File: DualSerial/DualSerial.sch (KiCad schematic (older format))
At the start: 22 parts, among them CN1 DB9 Male, CN2 DB9 Male, J1 COM_A_SELECT, J2 IRQ_A_SELECT, J3 COM_A_SELECT, J4 IRQ_B_SELECT, J5 Bus_ISA_8bit, U1 16550/16C550, U2 GAL16V8, U3 GD75232N, U4 1.8432 MHz, U8 16550/16C550, U9 GD75232N

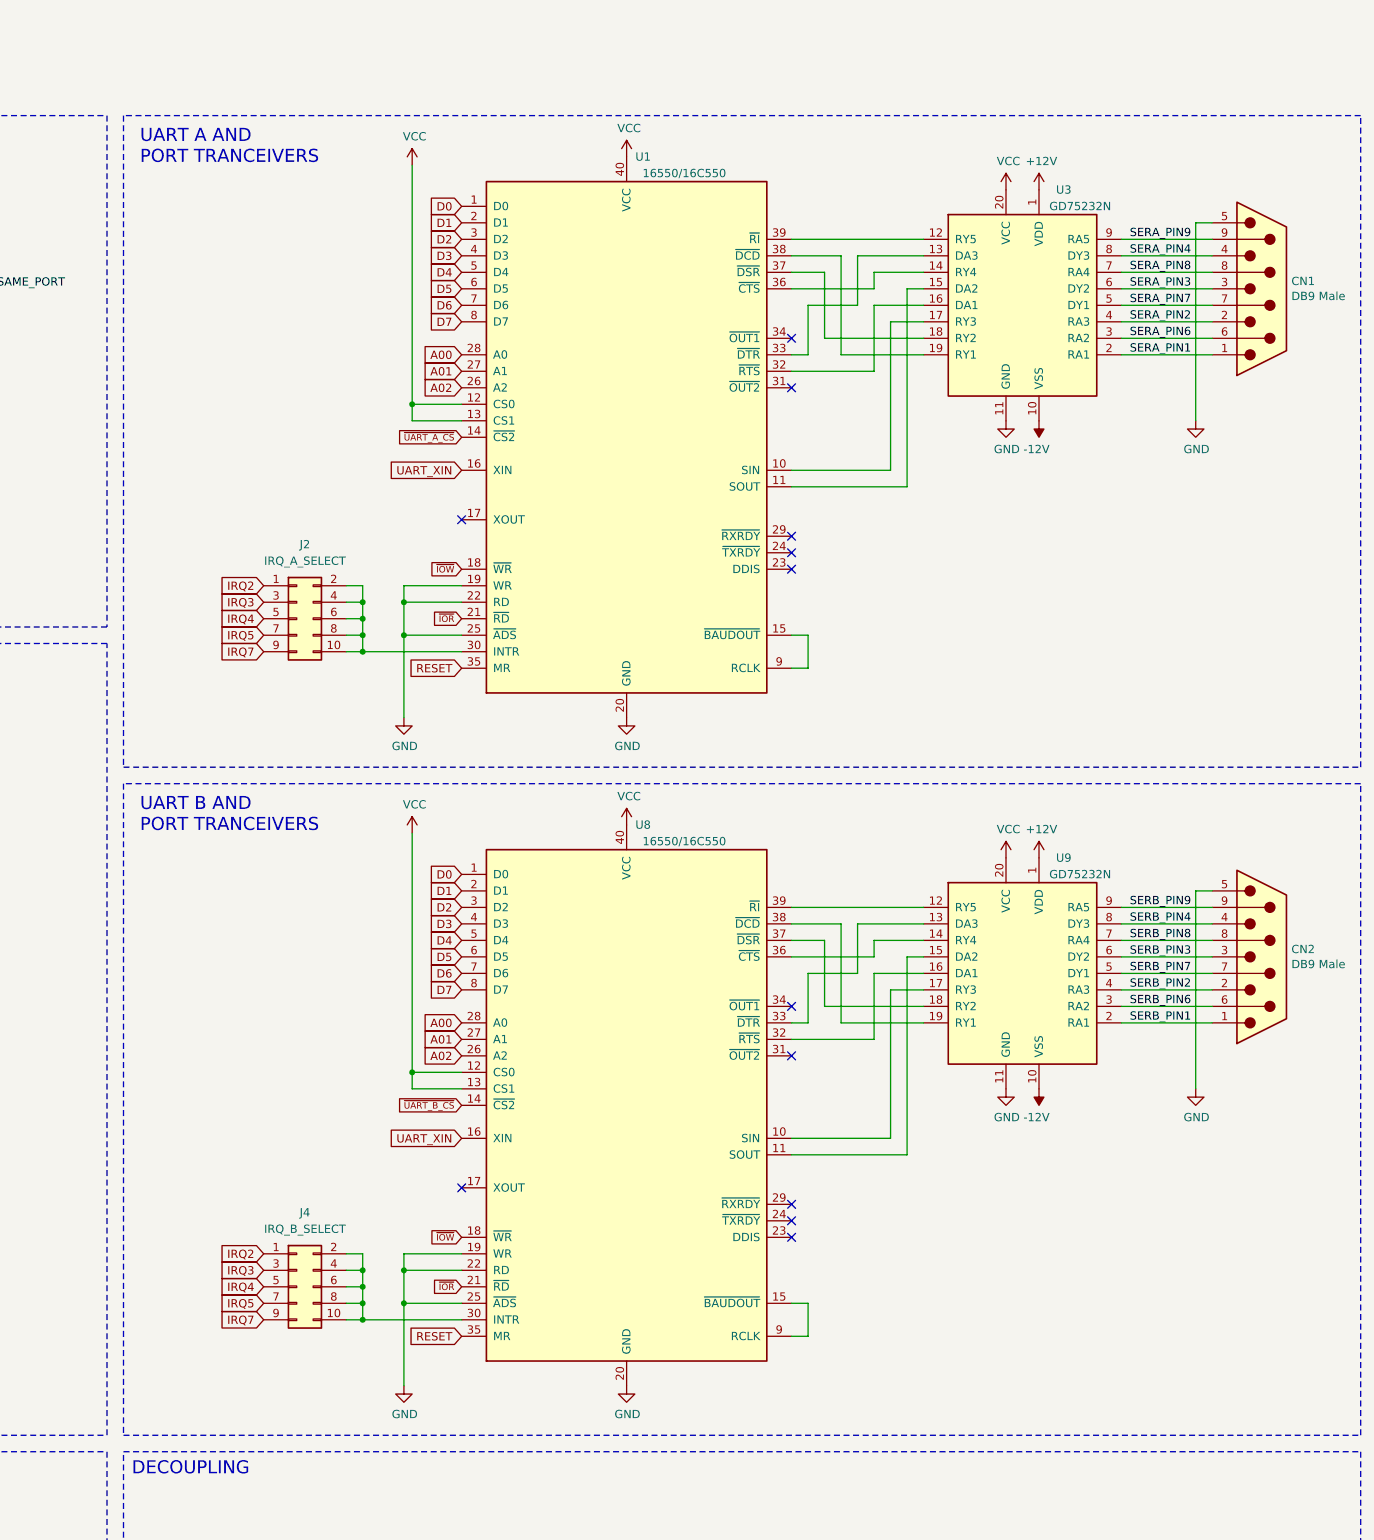
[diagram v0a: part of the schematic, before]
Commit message: DualSerial: More WIP on PCB layout.
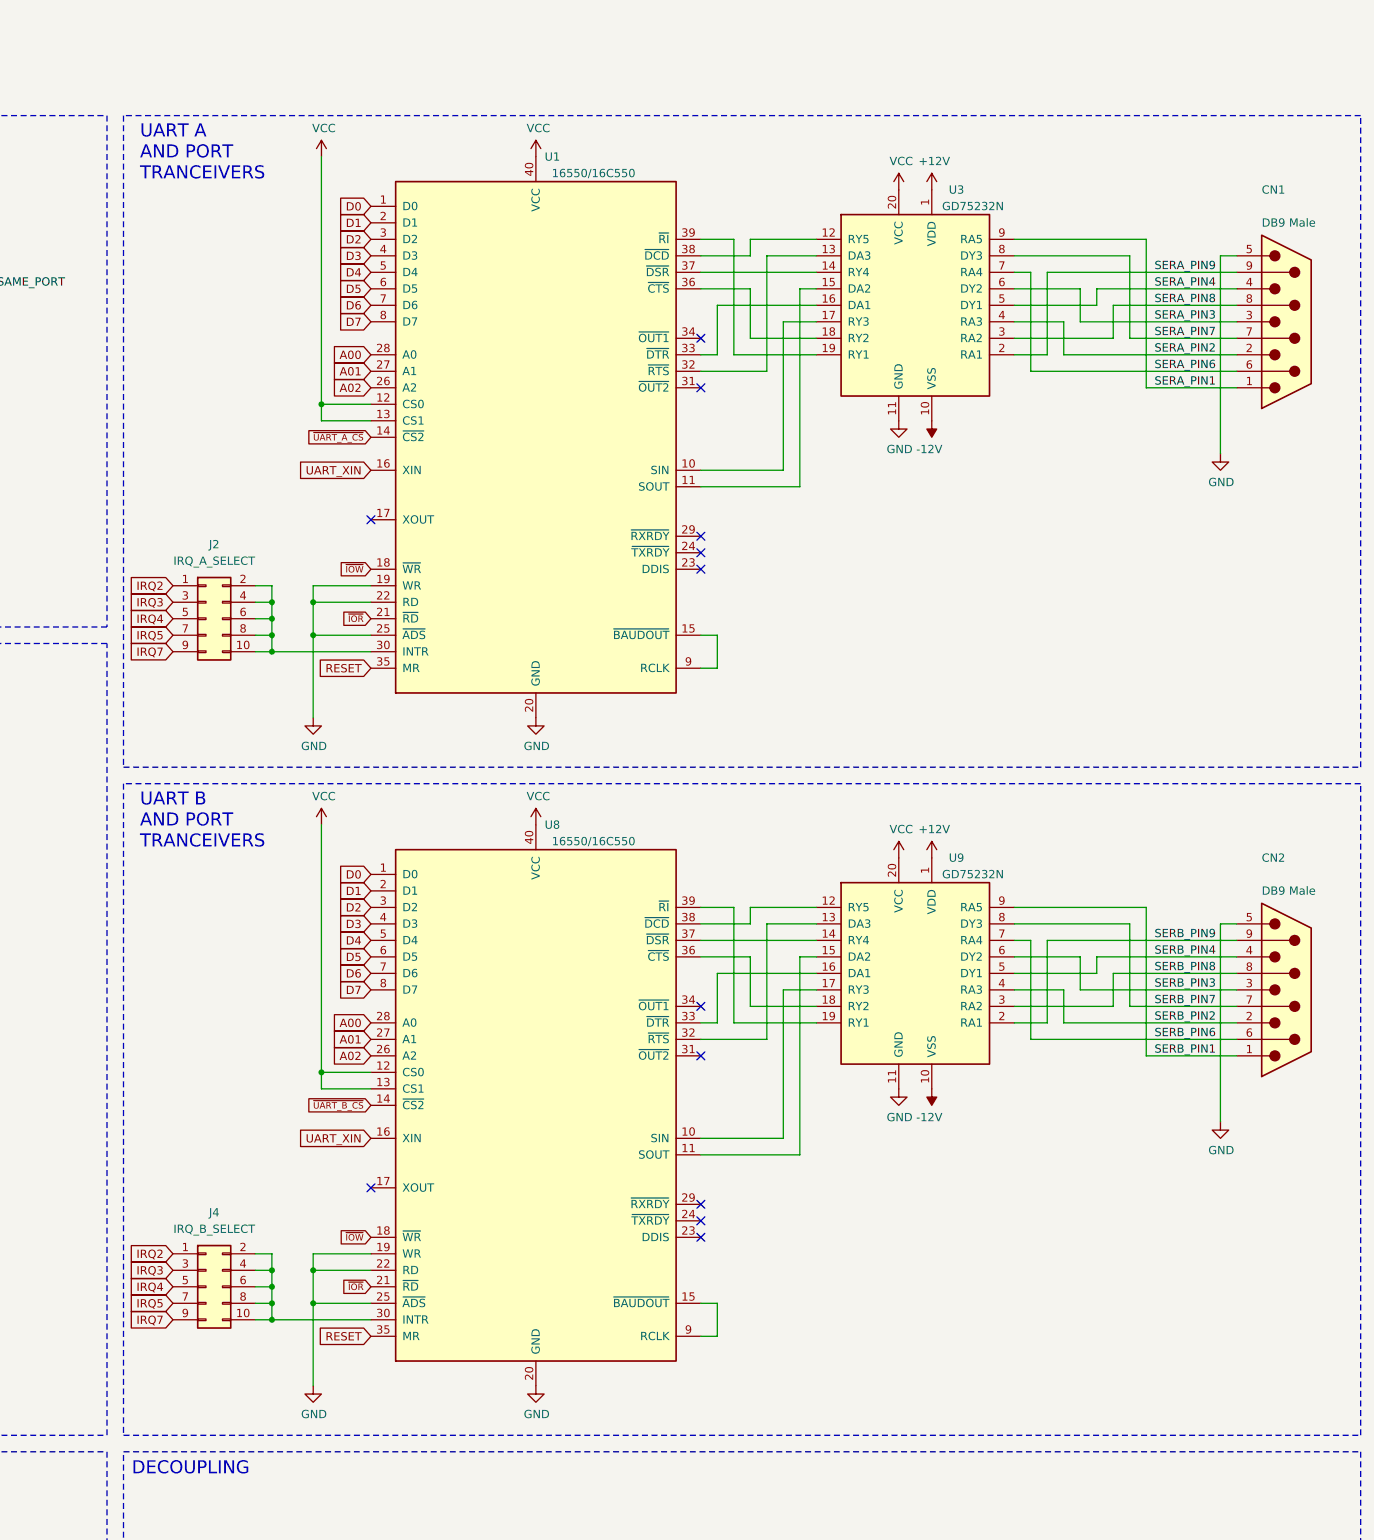
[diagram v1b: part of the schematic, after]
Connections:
- net SERA_PIN1: now also U3.9 (RA5); no longer U3.2 (RA1)
- net SERA_PIN4: now also U3.5 (DY1); no longer U3.8 (DY3)
- net SERA_PIN6: now also U3.7 (RA4); no longer U3.3 (RA2)
- net SERA_PIN7: now also U3.8 (DY3); no longer U3.5 (DY1)
- net SERA_PIN8: now also U3.3 (RA2); no longer U3.7 (RA4)
- net SERA_PIN9: now also U3.2 (RA1); no longer U3.9 (RA5)
- net SERB_PIN1: now also U9.9 (RA5); no longer U9.2 (RA1)
- net SERB_PIN4: now also U9.5 (DY1); no longer U9.8 (DY3)
- net SERB_PIN6: now also U9.7 (RA4); no longer U9.3 (RA2)
- net SERB_PIN7: now also U9.8 (DY3); no longer U9.5 (DY1)
- net SERB_PIN8: now also U9.3 (RA2); no longer U9.7 (RA4)
- net SERB_PIN9: now also U9.2 (RA1); no longer U9.9 (RA5)
- net at U1.32 (~RTS~): now also U3.13 (DA3); no longer U3.16 (DA1)
- net at U1.33 (~DTR~): now also U3.16 (DA1); no longer U3.13 (DA3)
- net at U1.36 (~CTS~): now also U3.18 (RY2); no longer U3.14 (RY4)
- net at U1.37 (~DSR~): now also U3.14 (RY4); no longer U3.18 (RY2)
- net at U1.38 (~DCD~): now also U3.12 (RY5); no longer U3.19 (RY1)
- net at U1.39 (~RI~): now also U3.19 (RY1); no longer U3.12 (RY5)
- net at U8.32 (~RTS~): now also U9.13 (DA3); no longer U9.16 (DA1)
- net at U8.33 (~DTR~): now also U9.16 (DA1); no longer U9.13 (DA3)
- net at U8.36 (~CTS~): now also U9.18 (RY2); no longer U9.14 (RY4)
- net at U8.37 (~DSR~): now also U9.14 (RY4); no longer U9.18 (RY2)
- net at U8.38 (~DCD~): now also U9.12 (RY5); no longer U9.19 (RY1)
- net at U8.39 (~RI~): now also U9.19 (RY1); no longer U9.12 (RY5)
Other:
- note added: "UART A\nAND PORT\nTRANCEIVERS"
- note added: "UART B\nAND PORT\nTRANCEIVERS"
- note removed: "UART A AND\nPORT TRANCEIVERS"
- note removed: "UART B AND\nPORT TRANCEIVERS"
- moved on the sheet: CN2, J2, J4, U1, U8, U9
